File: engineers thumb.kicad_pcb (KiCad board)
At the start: 2 copper layers, 47 x 81.3 mm, 57 parts, among them J1 Conn_01x01, J10 Conn_01x01, J11 Conn_01x01, J12 Conn_01x01, J13 Conn_01x01, J14 Conn_01x01, J15 Conn_01x01, J2 Conn_01x01, J3 Conn_01x01, J4 Conn_01x01, J5 Conn_01x01, J6 Conn_01x01, J7 Conn_01x01, J8 Conn_01x01, J9 Conn_01x01, Q1 Q_PMOS_GSD, Q2 BC327, U1 TL072, U2 TL072, U3 LM13700

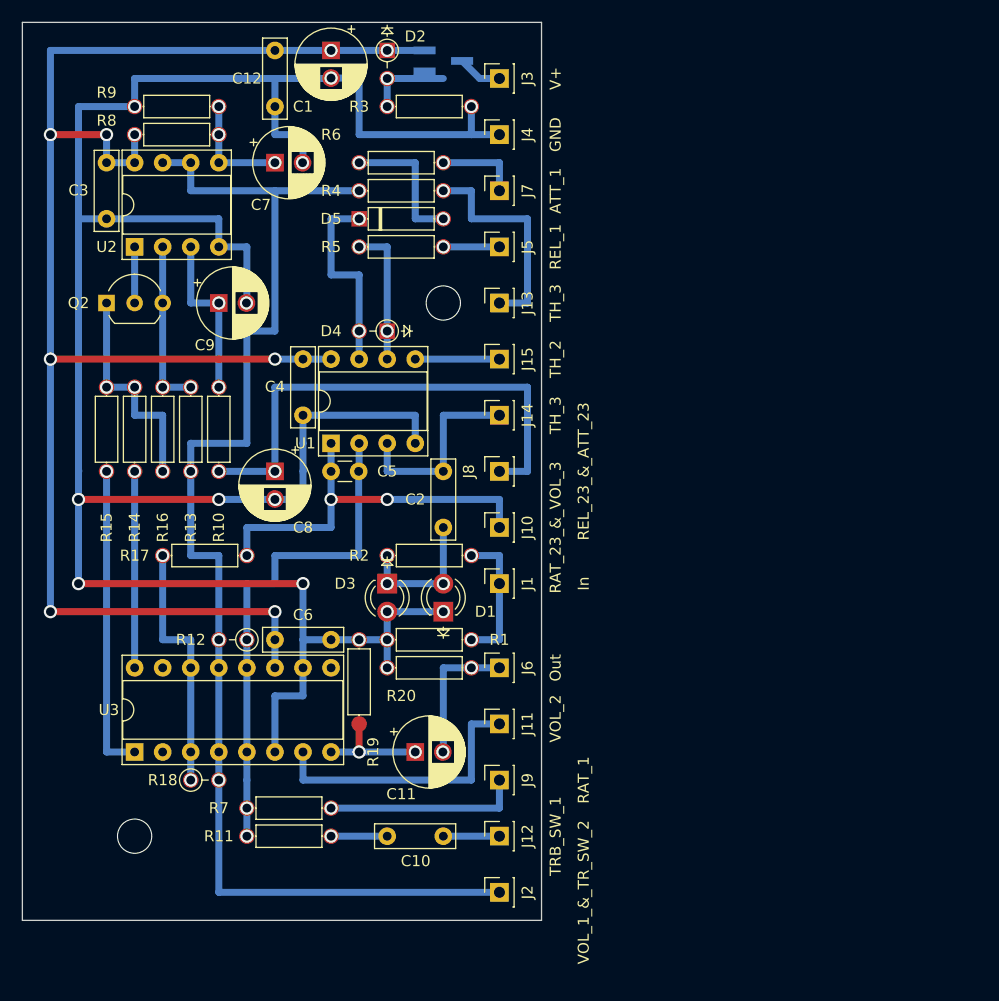
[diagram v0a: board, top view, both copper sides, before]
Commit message: its never done
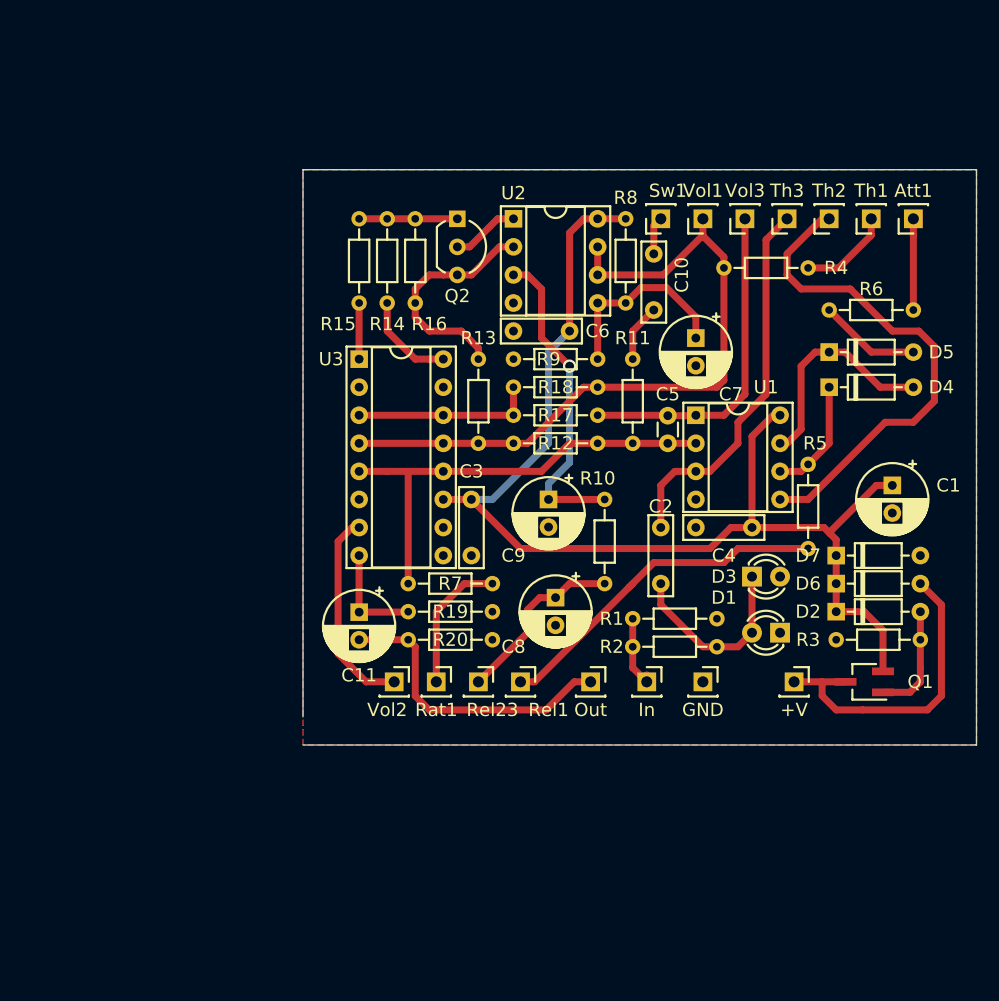
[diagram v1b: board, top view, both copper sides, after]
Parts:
- removed C12: 100n, 2.Breadboard components:C_Box_P5.08mm
- added D6: 1N4007, Diode_THT:D_DO-35_SOD27_P7.62mm_Horizontal, F.Cu at (109.2, 76.2)
- added D7: 1N4007, Diode_THT:D_DO-35_SOD27_P7.62mm_Horizontal, F.Cu at (109.2, 73.7)
- C1, C11, C7, C8, C9: footprint 2.Breadboard components:CP_Vertical -> Capacitor_THT:CP_Radial_D6.3mm_P2.50mm
- D1, D3: footprint 2.Breadboard components:LED_D3.0mm_Vertical -> LED_THT:LED_D3.0mm
- D2, D4: footprint 2.Breadboard components:D_Axial_Vertical -> Diode_THT:D_DO-35_SOD27_P7.62mm_Horizontal
- D5: footprint 2.Breadboard components:D_Axial_Horizontal -> Diode_THT:D_DO-35_SOD27_P7.62mm_Horizontal
- Q1: value Q_PMOS_GSD -> DMP3099L; moved to F.Cu
- R1, R10, R11, R13, R14, R15, R16, R17, R19, R2, R20, R3, R4, R5, R6, R7, R8, R9: footprint 2.Breadboard components:R_Axial_Horizontal -> Resistor_THT:R_Axial_DIN0204_L3.6mm_D1.6mm_P7.62mm_Horizontal
- R12, R18: footprint 2.Breadboard components:R_Axial_Vertical -> Resistor_THT:R_Axial_DIN0204_L3.6mm_D1.6mm_P7.62mm_Horizontal
- moved Q1 67.9 mm to (111.8, 85.1), turned to 180 degrees
- moved D2 65.1 mm to (109.2, 78.7), turned to 0 degrees
- moved C1 64.3 mm to (114.3, 67.3)
- moved J2 63.7 mm to (97.2, 43.2), turned to 180 degrees
- moved J3 60.8 mm to (105.4, 85.1), turned to 0 degrees
- moved R3 58.5 mm to (109.2, 81.3), turned to 0 degrees
- moved J12 57.8 mm to (93.3, 43.2), turned to 180 degrees
- moved C10 56.0 mm to (92.7, 46.4), turned to 270 degrees
- moved J4 52.8 mm to (97.2, 85.1), turned to 0 degrees
- moved R11 49.8 mm to (90.8, 63.5), turned to 90 degrees
- moved R18 46.0 mm to (80.0, 58.4)
- moved R5 45.2 mm to (106.7, 65.4), turned to 270 degrees
- moved C3 44.9 mm to (76.2, 68.6)
- moved R6 44.6 mm to (108.6, 51.4)
- moved D5 44.2 mm to (108.6, 55.2)
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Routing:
- net GND: track 221.1 -> 0.00 mm, vias 15 -> 0
- net +4V5: track 119.4 -> 64.3 mm, vias 4 -> 0
- net +9V: track 148.2 -> 107.5 mm, vias 9 -> 0
- net Net-(J15-Pad1): track 7.62 -> 45.6 mm
- net Net-(C8-Pad1): track 45.7 -> 16.3 mm, vias 2 -> 0
- net Net-(J5-Pad1): track 5.08 -> 31.5 mm, vias 1 -> 0
- net Net-(D6-Pad2): track 4.04 -> 28.7 mm
- net Net-(R15-Pad1): track 27.9 -> 5.08 mm, vias 1 -> 0
- net Net-(C2-Pad1): track 17.8 -> 34.5 mm
- net Net-(C11-Pad2): track 12.7 -> 27.2 mm, vias 2 -> 0
- net Net-(C9-Pad1): track 15.2 -> 29.0 mm, vias 2 -> 1
- net Net-(J13-Pad1): track 20.3 -> 8.43 mm, vias 1 -> 0
- net Net-(Q2-Pad1): track 20.3 -> 8.89 mm, vias 3 -> 0
- net Net-(R14-Pad1): track 17.8 -> 8.67 mm, vias 1 -> 0
- net Net-(C7-Pad1): track 10.2 -> 17.6 mm, vias 3 -> 0
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- added copper zone on B.Cu, net GND
- added copper zone on F.Cu, net GND
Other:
- board size 47 x 81.3 mm -> 61 x 52.1 mm

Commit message: Good progress made
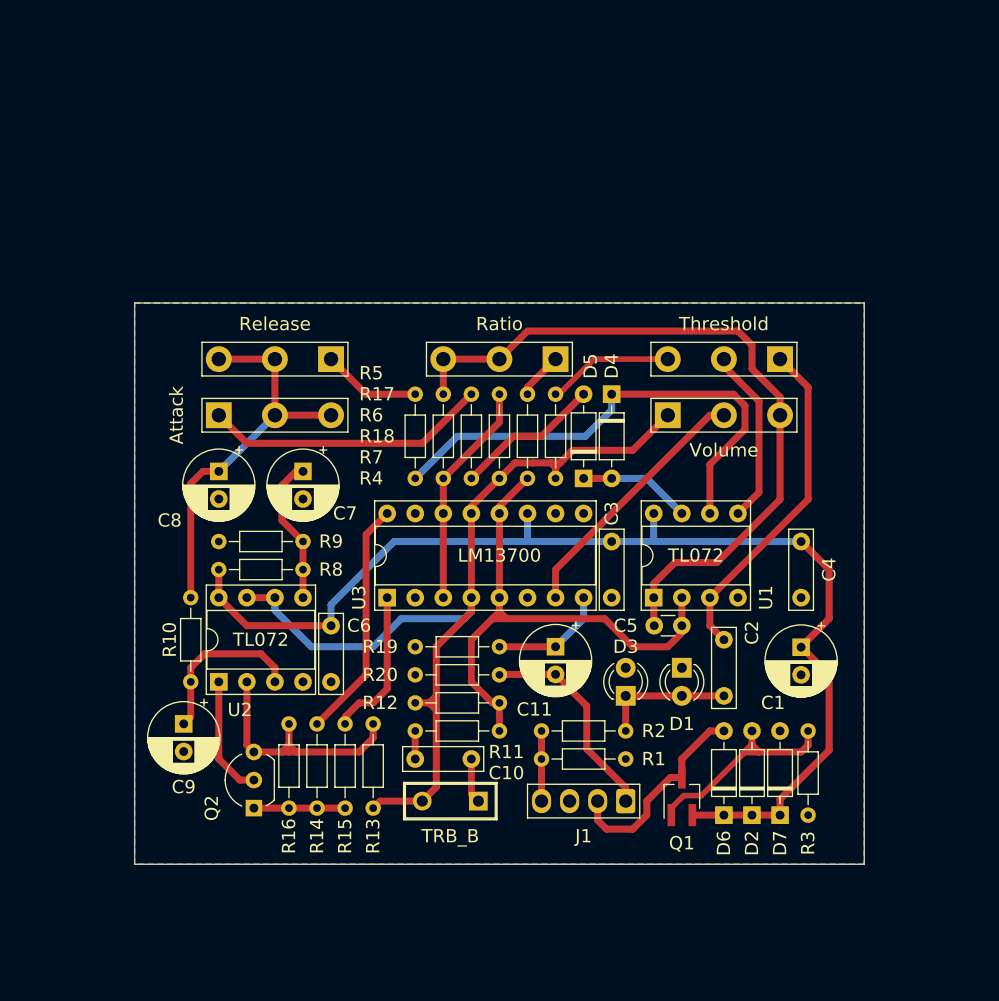
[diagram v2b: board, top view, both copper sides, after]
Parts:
- removed J10, J11, J12, J13, J14, J15, J2, J3, J4, J5, J6, J7, J8, J9: Conn_01x01, Connector_PinSocket_2.54mm:PinSocket_1x01_P2.54mm_Vertical
- added RV1: 1Meg_lin, 1.Custom footprints:Alpha_16mm_potentiometer, B.Cu at (99.1, 55.9)
- added RV2: 1Meg_log, 1.Custom footprints:Alpha_16mm_potentiometer, B.Cu at (78.7, 55.9)
- added RV3: 1Meg_lin, 1.Custom footprints:Alpha_16mm_potentiometer, B.Cu at (58.4, 55.9)
- added RV4: 100k_log, 1.Custom footprints:Alpha_16mm_potentiometer, B.Cu at (58.4, 61.0)
- added RV5: 10k_log, 1.Custom footprints:Alpha_16mm_potentiometer, B.Cu at (99.1, 61.0)
- added SW1: SPST, 1.Custom footprints:PinSocket_2x01_P2.54mm_Vertical_Wide, B.Cu at (76.8, 95.9)
- J1: value Conn_01x01 -> Conn_01x04_Female; footprint Connector_PinSocket_2.54mm:PinSocket_1x01_P2.54mm_Vertical -> 1.Custom footprints:Molex_KK-254_01x04_P2.54mm_Right_Angle
- moved Q2 56.4 mm to (56.5, 96.5), turned to 90 degrees
- moved R16 54.6 mm to (59.7, 96.5), turned to 90 degrees
- moved U2 49.7 mm to (53.3, 85.1), turned to 90 degrees
- moved C10 48.6 mm to (76.2, 92.1), turned to 180 degrees
- moved C9 38.8 mm to (50.2, 88.9)
- moved R14 38.6 mm to (62.2, 88.9), turned to 270 degrees
- moved R15 38.1 mm to (64.8, 88.9), turned to 270 degrees
- moved R8 37.9 mm to (61.0, 74.9), turned to 180 degrees
- moved C7 37.6 mm to (61.0, 66.0)
- moved R10 37.5 mm to (50.8, 77.5), turned to 270 degrees
- moved R6 35.8 mm to (76.2, 66.7), turned to 90 degrees
- moved R5 35.6 mm to (71.1, 66.7), turned to 90 degrees
- moved R13 34.4 mm to (67.3, 88.9)
- moved C6 34.3 mm to (63.5, 80.0), turned to 270 degrees
- moved C8 32.6 mm to (53.3, 66.0)
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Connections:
- C11 pad 2: Net-(C11-Pad2) -> Output
- D6 pad 2: Net-(D6-Pad2) -> Vin
- J1 pad 1: Net-(J1-Pad1) -> Output
- Q1 pad 3: Net-(D6-Pad2) -> Vin
- R1 pad 1: Net-(J1-Pad1) -> Input
- R2 pad 1: Net-(J1-Pad1) -> Input
- R20 pad 2: Net-(C11-Pad2) -> Output
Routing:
- net Net-(C5-Pad2): track 30.0 -> 66.1 mm
- net Net-(D4-Pad1): track 10.6 -> 45.3 mm
- net Net-(RV1-Pad2): track 45.6 -> 16.1 mm
- net Net-(D6-Pad2): track 28.7 -> 0.00 mm
- net Net-(C11-Pad2): track 27.2 -> 0.00 mm
- net Net-(R5-Pad2): track 31.5 -> 8.94 mm
- net +4V5: track 64.3 -> 85.1 mm
- net Net-(C8-Pad1): track 16.3 -> 35.7 mm
- net Output: track 0.00 -> 19.3 mm
- net Vin: track 0.00 -> 18.9 mm
- net Net-(R6-Pad2): track 8.26 -> 25.8 mm
- net Net-(C9-Pad1): track 29.0 -> 15.3 mm, vias 1 -> 0
- net Net-(R14-Pad1): track 8.67 -> 21.7 mm
- net Net-(D4-Pad2): track 20.1 -> 10.2 mm
- net Net-(D2-Pad2): track 10.1 -> 19.7 mm
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- added copper zone on F.Cu, net +9V
- removed copper zone on F.Cu, net GND
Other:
- board size 61 x 52.1 mm -> 66 x 50.8 mm
- net class Default: clearance 0.508 -> 0.381
- rule trace_clearance: 0.508 -> 0.381
- board text added: "LM13700"
- board text added: "TL072"
